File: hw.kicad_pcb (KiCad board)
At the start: 4 copper layers, 75 x 75 mm, 159 parts, among them IC2 ESDALC6V1W5, IC3 ESDALC6V1W5, IC4 QFN50P400X400X80-25N-D, IC5 QFN40P300X300X105-25N-D, J1 RECE.20279.001E.01, J2 RECE.20279.001E.01, J3 78800-0001, J4 AMPHENOL_10164227-1004A1RLF, J5 AMPHENOL_10164227-1004A1RLF, J7 USB4105-GF-A, Q1 BC847CE6327HTSA1, Q2 BC847CE6327HTSA1, Q3 BC847CE6327HTSA1, U11 XDFN8_1P7X1P3_ONS, U2 MOD100_LENA-R8_UBL, U3 STM32H745ZIT6, U4 XDFN8_1P7X1P3_ONS, U5 XDFN8_1P7X1P3_ONS, U8 TS3USB221RSER, Y1 NX3215SA-32.768K-EXS00A-MU000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, Y2 ATX-H11-F-25.000MHz-F25-T

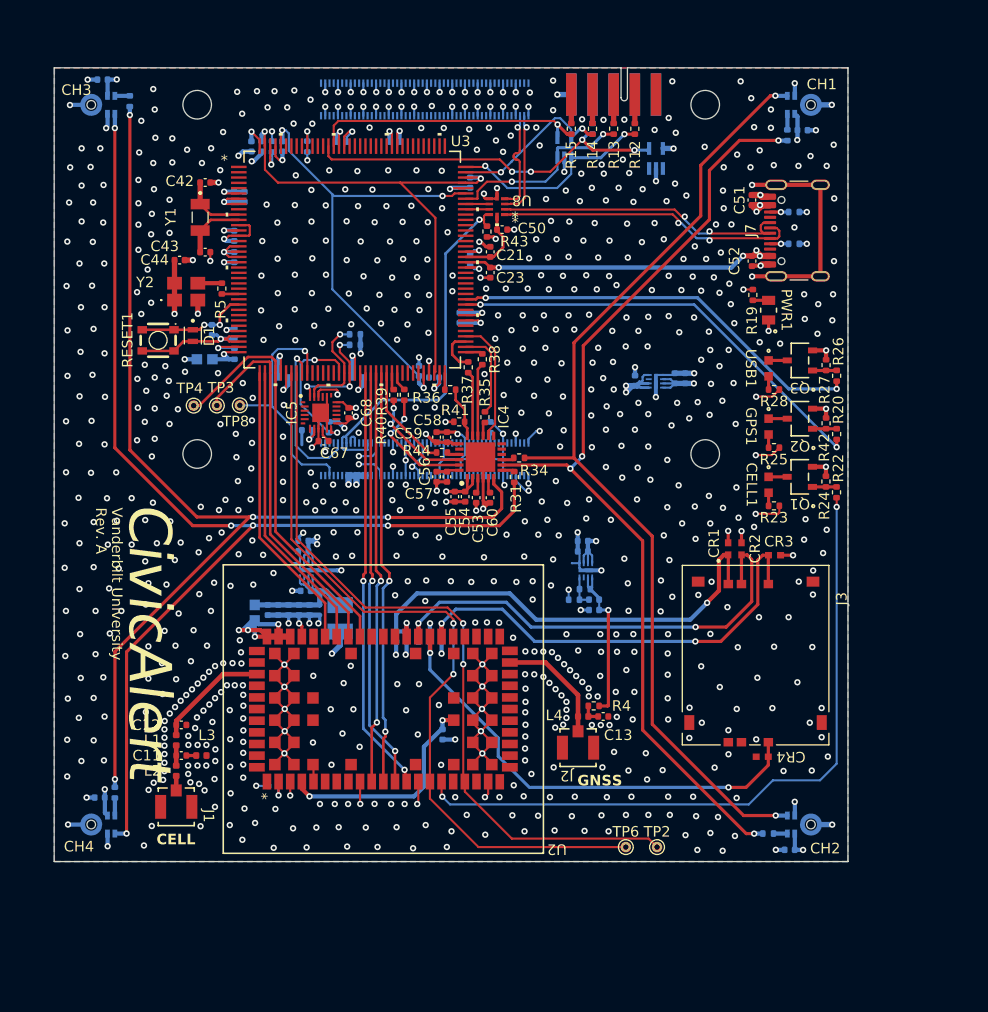
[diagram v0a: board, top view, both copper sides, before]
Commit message: Update for RevB
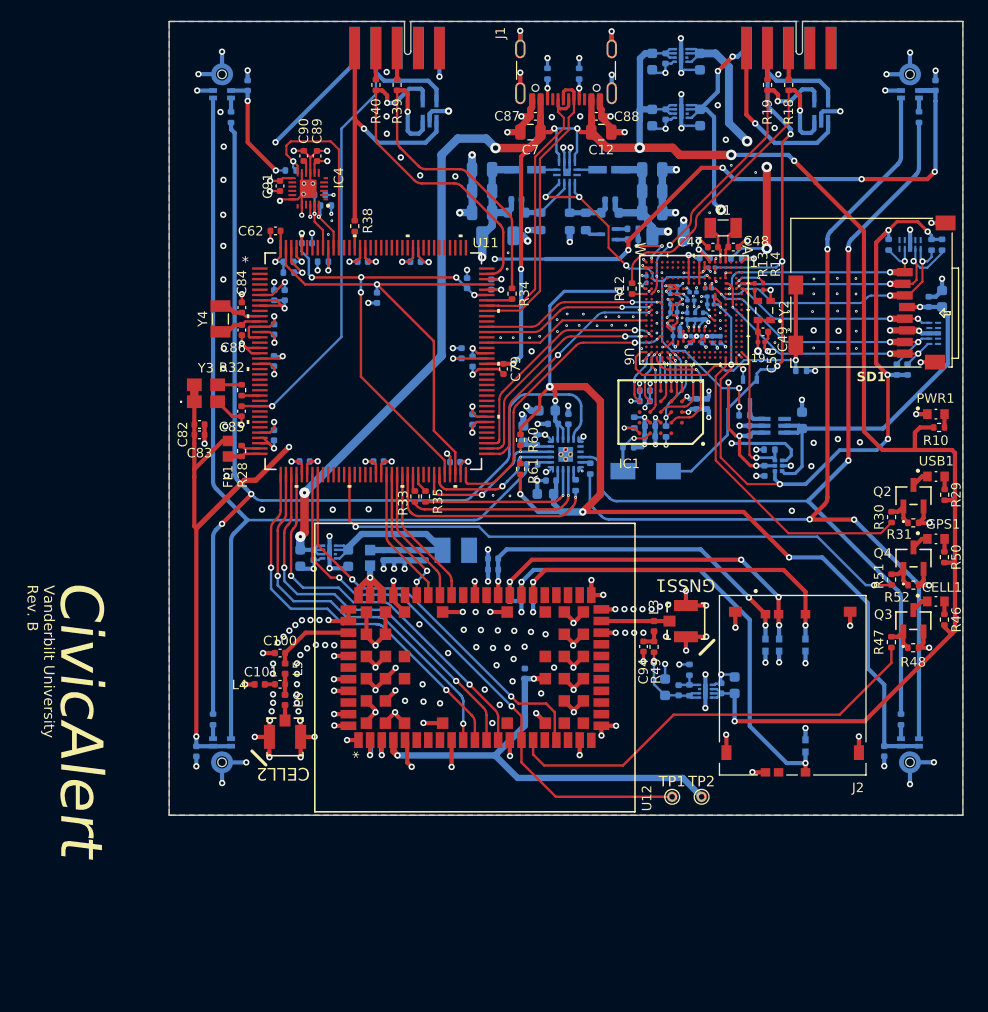
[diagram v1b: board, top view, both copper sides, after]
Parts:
- removed IC5: QFN40P300X300X105-25N-D, CivicAlert:ICM-20948
- removed J3: 78800-0001, CivicAlert:0788000001
- removed J4, J5: AMPHENOL_10164227-1004A1RLF, CivicAlert:10164227-1004A1RLF
- removed J7: USB4105-GF-A, Connector_USB:USB_C_Receptacle_GCT_USB4105-xx-A_16P_TopMnt_Horizontal
- removed Module1: ComputeModule5-CM5, CivicAlert:RPI-CM5IO
- removed RESET1: LS38G2-T, CivicAlert:LS38G2F-T
- removed TP3: GPS_TRIG, TestPoint:TestPoint_THTPad_D1.0mm_Drill0.5mm
- removed TP4: GPS_TP, TestPoint:TestPoint_THTPad_D1.0mm_Drill0.5mm
- removed TP6: GPS_PWR, TestPoint:TestPoint_THTPad_D1.0mm_Drill0.5mm
- removed TP8: RPI_nOFF, TestPoint:TestPoint_THTPad_D1.0mm_Drill0.5mm
- added B2: 009159010061911, CivicAlert:009159010061911, F.Cu at (137.5, 63.4)
- added C100: 1.5p, Capacitor_SMD:C_0402_1005Metric, F.Cu at (122.4, 120.5)
- added C101: 0.5p, Capacitor_SMD:C_0402_1005Metric, F.Cu at (122.4, 123.5)
- added C102: T520B337M006ATE040, CivicAlert:T520B337M006ATE040, B.Cu at (139.0, 110.8)
- added C103: 8.2p, Capacitor_SMD:C_0402_1005Metric, B.Cu at (132.2, 111.3)
- added C104: 15p, Capacitor_SMD:C_0402_1005Metric, B.Cu at (133.2, 111.3)
- added C105: 82p, Capacitor_SMD:C_0402_1005Metric, B.Cu at (134.2, 111.3)
- added C106: 10n, Capacitor_SMD:C_0402_1005Metric, B.Cu at (135.2, 111.3)
- added C107: 0.1u, Capacitor_SMD:C_0402_1005Metric, B.Cu at (136.2, 111.3)
- added C108: 0.1u, Capacitor_SMD:C_0402_1005Metric, B.Cu at (184.3, 66.9)
- added C109: 0.1u, Capacitor_SMD:C_0402_1005Metric, B.Cu at (179.5, 129.8)
- added C110: 0.1u, Capacitor_SMD:C_0402_1005Metric, B.Cu at (119.4, 66.9)
- added C111: 0.1u, Capacitor_SMD:C_0402_1005Metric, B.Cu at (114.5, 129.8)
- added C112: 0.1u, Capacitor_SMD:C_0402_1005Metric, B.Cu at (148.2, 98.9)
- added C113: 10u, Capacitor_SMD:C_0603_1608Metric, B.Cu at (147.6, 97.6)
- added C114: 2.2u, Capacitor_SMD:C_0402_1005Metric, B.Cu at (149.7, 98.4)
- added C115: 10u, Capacitor_SMD:C_0603_1608Metric, B.Cu at (147.5, 105.5)
- added C116: 0.1u, Capacitor_SMD:C_0402_1005Metric, B.Cu at (148.0, 104.2)
- added C117: 0.1u, Capacitor_SMD:C_0402_1005Metric, B.Cu at (146.7, 100.4)
- added C118: 10u, Capacitor_SMD:C_0603_1608Metric, B.Cu at (145.4, 99.8)
- added C70: 0.1u, Capacitor_SMD:C_0402_1005Metric, B.Cu at (124.7, 102.4)
- added C71: 0.1u, Capacitor_SMD:C_0402_1005Metric, B.Cu at (131.7, 102.4)
- added C72: 0.1u, Capacitor_SMD:C_0402_1005Metric, B.Cu at (139.0, 102.5)
- added C73: 0.1u, Capacitor_SMD:C_0402_1005Metric, B.Cu at (140.6, 98.5)
- added C74: 0.1u, Capacitor_SMD:C_0402_1005Metric, B.Cu at (140.6, 93.0)
- added C75: 0.1u, Capacitor_SMD:C_0402_1005Metric, B.Cu at (142.4, 85.7)
- added C76: 4.7u, Capacitor_SMD:C_0402_1005Metric, B.Cu at (131.6, 87.0)
- added C77: 0.1u, Capacitor_SMD:C_0402_1005Metric, B.Cu at (122.9, 86.7)
- added C78: 2.2u, Capacitor_SMD:C_0402_1005Metric, B.Cu at (139.6, 92.2)
- added C79: 4.7u, Capacitor_SMD:C_0402_1005Metric, F.Cu at (143.5, 93.7)
- added C80: 2.2u, Capacitor_SMD:C_0402_1005Metric, B.Cu at (125.0, 81.8)
- added C81: 2.2u, Capacitor_SMD:C_0402_1005Metric, B.Cu at (140.1, 85.6)
- added C82: 10n, Capacitor_SMD:C_0402_1005Metric, F.Cu at (114.8, 98.9)
- added C83: 0.1u, Capacitor_SMD:C_0402_1005Metric, F.Cu at (114.8, 99.9)
- added C84: 3.3p, Capacitor_SMD:C_0402_1005Metric, F.Cu at (118.8, 87.9)
- added C85: 0.1u, Capacitor_SMD:C_0402_1005Metric, F.Cu at (118.8, 97.7)
- added C86: 3.3p, Capacitor_SMD:C_0402_1005Metric, F.Cu at (118.8, 90.0)
- added C87: 0.1u, Capacitor_SMD:C_0402_1005Metric, F.Cu at (146.5, 69.8)
- added C88: 0.1u, Capacitor_SMD:C_0402_1005Metric, F.Cu at (152.3, 69.8)
- added C89: 0.1u, Capacitor_SMD:C_0402_1005Metric, F.Cu at (125.9, 73.6)
- added C9: 10u, Capacitor_SMD:C_0805_2012Metric, B.Cu at (141.5, 78.9)
- added C90: 0.1u, Capacitor_SMD:C_0402_1005Metric, F.Cu at (124.6, 73.6)
- added C91: 0.1u, Capacitor_SMD:C_0402_1005Metric, F.Cu at (122.4, 76.4)
- added C92: 0.1u, Capacitor_SMD:C_0402_1005Metric, B.Cu at (131.5, 129.1)
- added C93: 0.1u, Capacitor_SMD:C_0402_1005Metric, B.Cu at (145.5, 122.5)
- added C94: 0.1u, Capacitor_SMD:C_0402_1005Metric, F.Cu at (156.7, 119.9)
- added C95: 47p, Capacitor_SMD:C_0402_1005Metric, B.Cu at (146.3, 115.1)
- added C96: 47p, Capacitor_SMD:C_0402_1005Metric, B.Cu at (145.2, 115.1)
- added C97: 47p, Capacitor_SMD:C_0402_1005Metric, B.Cu at (144.1, 115.1)
- added C98: 47p, Capacitor_SMD:C_0402_1005Metric, B.Cu at (142.5, 111.6)
- added C99: 0.1u, Capacitor_SMD:C_0402_1005Metric, B.Cu at (142.5, 112.7)
- added CELL2: RECE.20279.001E.01, CivicAlert:RECE.20279.001E.01, F.Cu at (122.9, 128.5)
- added CR5: PESD0402-140, CivicAlert:PESD0402-140_LTF, B.Cu at (172.1, 119.8)
- added GNSS1: RECE.20279.001E.01, CivicAlert:RECE.20279.001E.01, F.Cu at (160.8, 117.5)
- added IC1: MX25UM25645GXDI00-T, CivicAlert:MX25UM25645GXDI00, F.Cu at (158.4, 97.8)
- added L5: 2.7n, Inductor_SMD:L_0402_1005Metric, F.Cu at (122.9, 122.0)
- added L6: 1.2n, Inductor_SMD:L_0402_1005Metric, F.Cu at (122.9, 125.0)
- added Q4: MMBT3904LT3G, CivicAlert:MMBT3904LT3G, F.Cu at (182.3, 111.6)
- added R16: 10k, Resistor_SMD:R_0402_1005Metric, B.Cu at (155.9, 98.8)
- added R17: 10k, Resistor_SMD:R_0402_1005Metric, B.Cu at (158.9, 99.6)
- added R46: 300, Resistor_SMD:R_0402_1005Metric, F.Cu at (185.2, 117.4)
- added R47: 10k, Resistor_SMD:R_0402_1005Metric, F.Cu at (180.2, 119.5)
- added R48: 47k, Resistor_SMD:R_0402_1005Metric, F.Cu at (182.2, 120.0)
- added R49: 33, Resistor_SMD:R_0402_1005Metric, F.Cu at (157.7, 120.0)
- added R50: 300, Resistor_SMD:R_0402_1005Metric, F.Cu at (185.2, 111.5)
- added R51: 10k, Resistor_SMD:R_0402_1005Metric, F.Cu at (180.2, 113.6)
- added R52: 47k, Resistor_SMD:R_0402_1005Metric, F.Cu at (182.2, 114.1)
- added R53: 47, Resistor_SMD:R_0402_1005Metric, B.Cu at (182.8, 69.9)
- added R54: 47, Resistor_SMD:R_0402_1005Metric, B.Cu at (181.1, 126.8)
- added R55: 47, Resistor_SMD:R_0402_1005Metric, B.Cu at (117.8, 69.9)
- added R56: 47, Resistor_SMD:R_0402_1005Metric, B.Cu at (116.1, 126.8)
- added R57: 47, Resistor_SMD:R_0402_1005Metric, B.Cu at (150.3, 104.7)
- added R58: 22, Resistor_SMD:R_0402_1005Metric, B.Cu at (146.2, 102.7)
- added R59: 22, Resistor_SMD:R_0402_1005Metric, B.Cu at (151.7, 103.1)
- added R60: 10k, Resistor_SMD:R_0402_1005Metric, F.Cu at (145.1, 100.4)
- added R61: 10k, Resistor_SMD:R_0402_1005Metric, F.Cu at (145.1, 103.1)
- added SD1: 15882, CivicAlert:15882, F.Cu at (178.3, 86.5)
- added TP1: GPS_PWR, TestPoint:TestPoint_THTPad_D1.0mm_Drill0.5mm, F.Cu at (159.5, 134.1)
- added U1: LTC3315AHV-TRMPBF, CivicAlert:LTC3315AHV, B.Cu at (149.5, 75.1)
- added U10: TPS22919DCKR, CivicAlert:TPS22919DCKR, B.Cu at (169.1, 99.1)
- added U12: LENA-R8001M10-00C, CivicAlert:LENA-R8001M10-00C, F.Cu at (140.8, 121.9)
- added U13: PCMD3140IRTER, CivicAlert:PCMD3140IRTER, B.Cu at (149.4, 101.8)
- added U6: STM32N647L0H3Q, CivicAlert:STM32N647L0H3Q, F.Cu at (161.5, 88.1)
- added U7: HSP051-4M10, CivicAlert:HSP051-4M10, B.Cu at (181.9, 81.9)
- added U9: NX3L1T3157GMZ, CivicAlert:NX3L1T3157GMZ, B.Cu at (169.5, 102.8)
- added Y3: ATX-H11-F-25.000MHz-F25-T, CivicAlert:ATX-H11-F-25_000MHz-F25-T, F.Cu at (115.4, 96.0)
- added Y4: ABS07AIG-32.768KHZ-7-T, CivicAlert:ABS07AIG_32_768KHZ_7_T, F.Cu at (116.8, 89.0)
- C1: value 100n -> 6.8p
- C10, C3: value 100n -> 10u; footprint Capacitor_SMD:C_0402_1005Metric -> Capacitor_SMD:C_0805_2012Metric
- C11: value 0.5p -> 10u; footprint Capacitor_SMD:C_0402_1005Metric -> Capacitor_SMD:C_0805_2012Metric; moved to B.Cu
- C12: value 1.5p -> 10u; footprint Capacitor_SMD:C_0402_1005Metric -> Capacitor_SMD:C_0805_2012Metric
- C13: value 100n -> 1n; moved to B.Cu
- C14, C15, C17: value 47p -> 10u; footprint Capacitor_SMD:C_0402_1005Metric -> Capacitor_SMD:C_0603_1608Metric
- C16: value 47p -> 0.1u
- C18, C24, C64: value 100n -> 0.1u
- C19, C20: value 2.2u -> 10u; footprint Capacitor_SMD:C_0402_1005Metric -> Capacitor_SMD:C_0603_1608Metric
- C2: value 100n -> 4.7p
- C21: value 2.2u -> 0.1u; moved to B.Cu
- C22: value 4.7u -> 10u; footprint Capacitor_SMD:C_0402_1005Metric -> Capacitor_SMD:C_0603_1608Metric
- C23: value 4.7u -> 10u; footprint Capacitor_SMD:C_0402_1005Metric -> Capacitor_SMD:C_0603_1608Metric; moved to B.Cu
- C25, C61: value 100n -> 10u; footprint Capacitor_SMD:C_0402_1005Metric -> Capacitor_SMD:C_0603_1608Metric
- C26, C27, C28, C29, C31, C32, C33, C34, C35, C36, C37, C46: value 100n -> 0.1u; footprint Capacitor_SMD:C_0402_1005Metric -> Capacitor_SMD:C_0201_0603Metric
- C30, C41: value 100n -> 2.2u; footprint Capacitor_SMD:C_0402_1005Metric -> Capacitor_SMD:C_0201_0603Metric
- C38: value 4.7u -> 0.1u; footprint Capacitor_SMD:C_0402_1005Metric -> Capacitor_SMD:C_0201_0603Metric
- C39, C40: value 10u -> 2.2u; footprint Capacitor_SMD:C_0402_1005Metric -> Capacitor_SMD:C_0201_0603Metric
- C4: value 8.2p -> 10u; footprint Capacitor_SMD:C_0402_1005Metric -> Capacitor_SMD:C_0805_2012Metric
- C42, C43: value 1.5p -> 2.2u; footprint Capacitor_SMD:C_0402_1005Metric -> Capacitor_SMD:C_0201_0603Metric; moved to B.Cu
- C44: value 10n -> 4.7u; moved to B.Cu
- C45: value 10u -> 0.1u; footprint Capacitor_SMD:C_0402_1005Metric -> Capacitor_SMD:C_0201_0603Metric
- C47: value 10u -> 3.3p; moved to F.Cu
- C48: value 100n -> 3.3p; moved to F.Cu
- C49: value 100n -> 10n; moved to F.Cu
- C5: value 15p -> 10u; footprint Capacitor_SMD:C_0402_1005Metric -> Capacitor_SMD:C_0805_2012Metric
- C50: value 2.2u -> 0.1u; footprint Capacitor_SMD:C_0402_1005Metric -> Capacitor_SMD:C_0201_0603Metric
- C51, C54, C57, C67, C68: value 100n -> 0.1u; moved to B.Cu
- C52: value 100n -> 4.7u; moved to B.Cu
- C53: value 2.2u -> 4.7u; moved to B.Cu
- C55, C59: value 10u -> 0.1u; moved to B.Cu
- C56: value 10u -> 4.7u; moved to B.Cu
- C58: value 100n -> 10u; footprint Capacitor_SMD:C_0402_1005Metric -> Capacitor_SMD:C_0603_1608Metric; moved to B.Cu
- C6: value 82p -> 47u; footprint Capacitor_SMD:C_0402_1005Metric -> Capacitor_SMD:C_1206_3216Metric
- C60, CR2, CR3, CR4, R24: moved to B.Cu
- C62: value 100n -> 4.7u; moved to F.Cu
- C63, C65: value 10u -> 0.1u
- C66: value 1n -> 0.1u
- C69: value T520B337M006ATE040 -> 0.1u; footprint CivicAlert:T520B337M006ATE040 -> Capacitor_SMD:C_0402_1005Metric
- C7: value 10n -> 10u; footprint Capacitor_SMD:C_0402_1005Metric -> Capacitor_SMD:C_0805_2012Metric; moved to F.Cu
- C8: value 100n -> 47u; footprint Capacitor_SMD:C_0402_1005Metric -> Capacitor_SMD:C_1206_3216Metric
- CELL1, GPS1, USB1: value LTST-C193TBKT-5A -> LTST-C190KGKT; footprint CivicAlert:LTST-C193TBKT-5A -> CivicAlert:LTST-C190KGKT
- CR1: value PESD0402-140 -> BAT854AW; footprint CivicAlert:PESD0402-140_LTF -> CivicAlert:BAT854AW,115; moved to B.Cu
- D1: value NSPM2051MUT5G -> B140Q-13-F; footprint CivicAlert:NSPM2051MUT5G -> CivicAlert:B140Q-13-F; moved to B.Cu
- FL1: value BLM18EG221SN1D -> FCM 1608KF-601T03; footprint CivicAlert:BLM18EG221SN1D -> CivicAlert:FCM1608KF-601T03; moved to F.Cu
- FL2: value FCM 1608KF-601T03 -> BLM18EG221SN1D; footprint CivicAlert:FCM1608KF-601T03 -> CivicAlert:BLM18EG221SN1D
- IC4: value QFN50P400X400X80-25N-D -> ICM-20948; footprint CivicAlert:PCMD3180IRTWT -> CivicAlert:ICM-20948
- J1: value RECE.20279.001E.01 -> USB4105-GF-A; footprint CivicAlert:RECE.20279.001E.01 -> Connector_USB:USB_C_Receptacle_GCT_USB4105-xx-A_16P_TopMnt_Horizontal
- J2: value RECE.20279.001E.01 -> 78800-0001; footprint CivicAlert:RECE.20279.001E.01 -> CivicAlert:0788000001
- L1: value 2.7n -> IHLP1212BZERR88M11; footprint Inductor_SMD:L_0402_1005Metric -> CivicAlert:IHLP1212BZERR88M11; moved to B.Cu
- L2: value 1.2n -> IHLP1212BZER1R5M11; footprint Inductor_SMD:L_0402_1005Metric -> CivicAlert:IHLP1212BZER1R5M11; moved to B.Cu
- L3: value 3.4n -> 120n
- L4: value 120n -> 3.4n
- PWR1: value LTST-C170KRKT -> LTST-C190KGKT; footprint CivicAlert:LTST-C170KRKT -> CivicAlert:LTST-C190KGKT
- Q1: value BC847CE6327HTSA1 -> SI1062X-T1-GE3; footprint CivicAlert:BC847CE6327HTSA1 -> CivicAlert:SI1062X-T1-GE3; moved to B.Cu
- Q2, Q3: value BC847CE6327HTSA1 -> MMBT3904LT3G; footprint CivicAlert:BC847CE6327HTSA1 -> CivicAlert:MMBT3904LT3G
- R1: value 50 -> 1M
- R10: value 10k -> 300; moved to F.Cu
- R13: footprint Resistor_SMD:R_0402_1005Metric -> Resistor_SMD:R_0201_0603Metric
- R14: value 22 -> 1k; footprint Resistor_SMD:R_0402_1005Metric -> Resistor_SMD:R_0201_0603Metric
- R15: value 22 -> 10k; moved to B.Cu
- R18: moved to F.Cu
- R19: value 250 -> 22
- R2: value 50 -> 150k
- R20, R22: value 10k -> 47k; moved to B.Cu
- R21: value 8.2k -> 10k
- R23, R25: value 500 -> 47k; moved to B.Cu
- R26: value 10k -> 100k; moved to B.Cu
- R27: value 47k -> 10k; moved to B.Cu
- R28: value 500 -> 47
- R29: value 5.1k -> 300; moved to F.Cu
- R3: value 50 -> 226k; footprint Resistor_SMD:R_0402_1005Metric -> Resistor_SMD:R_0603_1608Metric
- R30: value 5.1k -> 10k; moved to F.Cu
- R31: value 22 -> 47k
- R32: value 50 -> 22; moved to F.Cu
- R33: value 50 -> 47; moved to F.Cu
- R35: value 50 -> 47
- R36, R37, R44: value 50 -> 10k; moved to B.Cu
- R38, R39, R40: value 50 -> 22
- R4: value 33 -> 887k; footprint Resistor_SMD:R_0402_1005Metric -> Resistor_SMD:R_0603_1608Metric; moved to B.Cu
- R41: value 10k -> 5.1k; moved to B.Cu
- R42: value 47k -> 5.1k; moved to B.Cu
- R43: value 100k -> 10k; moved to B.Cu
- R45: value 1k -> 10k
- R5: value 50 -> 140k; footprint Resistor_SMD:R_0402_1005Metric -> Resistor_SMD:R_0603_1608Metric; moved to B.Cu
- R6: value 5.1k -> 97.6k; footprint Resistor_SMD:R_0402_1005Metric -> Resistor_SMD:R_0603_1608Metric
- R7: value 10k -> 261k; footprint Resistor_SMD:R_0402_1005Metric -> Resistor_SMD:R_0603_1608Metric
- R8: value 10k -> 62k
- R9: value 10k -> 91k
- TP2: value GPS_nRST -> GPS_VINT
- U11: value XDFN8_1P7X1P3_ONS -> STM32H745ZIT6; footprint CivicAlert:NCP186BMX185TAG -> CivicAlert:STM32H745ZIT6; moved to F.Cu
- U2: value MOD100_LENA-R8_UBL -> NCP186AMX180TAG; footprint CivicAlert:LENA-R8001M10-00C -> CivicAlert:NCP186AMX; moved to B.Cu
- U3: value STM32H745ZIT6 -> NCP186AMX390TAG; footprint CivicAlert:STM32H745ZIT6 -> CivicAlert:NCP186AMX; moved to B.Cu
- U4: value XDFN8_1P7X1P3_ONS -> NCP186AMX180TAG; footprint CivicAlert:NCP186AMX390TAG -> CivicAlert:NCP186AMX
- U5: value XDFN8_1P7X1P3_ONS -> NCP186AMX330TAG; footprint CivicAlert:NCP186BMX185TAG -> CivicAlert:NCP186AMX
- U8: value TS3USB221RSER -> HSP051-4M10; footprint CivicAlert:TS3USB221RSER -> CivicAlert:HSP051-4M10; moved to B.Cu
- Y1: value NX3215SA-32.768K-EXS00A-MU00003 -> ABS07AIG-32.768KHZ-7-T; footprint CivicAlert:NX3215SA-32_768K-EXS00A-MU0000 -> CivicAlert:ABS07AIG_32_768KHZ_7_T
- Y2: value ATX-H11-F-25.000MHz-F25-T -> KC2016Z48.0000C15XXK; footprint CivicAlert:ATX-H11-F-25_000MHz-F25-T -> CivicAlert:KC2016Z48.0000C15XXK
- moved J1 79.6 mm to (149.4, 64.5)
- moved C61 73.5 mm to (171.7, 98.5), turned to 90 degrees
- moved C12 68.6 mm to (152.8, 71.3)
- moved L1 67.7 mm to (153.5, 74.9), turned to 0 degrees
- moved C2 66.7 mm to (144.7, 77.7)
- moved L2 65.7 mm to (145.6, 74.9), turned to 180 degrees
- moved R10 65.3 mm to (184.7, 99.2), turned to 180 degrees
- moved C11 62.2 mm to (141.5, 74.9)
- moved U4 60.2 mm to (160.3, 64.1), turned to 180 degrees
- moved C10 59.6 mm to (141.5, 76.9)
- moved R2 58.5 mm to (155.8, 80.5)
- moved C62 56.1 mm to (122.0, 80.7), turned to 0 degrees
- moved Y2 54.6 mm to (168.2, 88.2), turned to 180 degrees
- moved C5 54.6 mm to (157.6, 74.9), turned to 0 degrees
- moved C4 53.7 mm to (157.6, 76.9), turned to 0 degrees
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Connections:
- B1 pad 10: MCU_VCC -> VCC_AI_IO
- B1 pad 2: Net-(B1-JTDI) -> unconnected-(B1-JTDI-Pad2)
- B1 pad 5: Net-(B1-JTDO/SWO) -> AI_SWO
- B1 pad 9: Net-(B1-NRST) -> AI_NRST
- C1 pad 1: MCU_VCC -> Net-(U1-FB1)
- C1 pad 2: GND -> VCC_AI_CORE
- C10 pad 1: Net-(U2-V_BCKP) -> VCC_MCU
- C11 pad 1: Net-(C11-Pad1) -> VCC_MCU
- C11 pad 2: Net-(C11-Pad2) -> GND
- C12 pad 2: Net-(U2-ANT) -> VCC_5V
- C13 pad 1: GND -> VCC_GPS_ANT
- C13 pad 2: Net-(C13-Pad2) -> Net-(U2-FB/ADJ)
- C14 pad 1: GND -> VCC_GPS_ANT
- C14 pad 2: SIM_CLK -> GND
- C15 pad 1: GND -> VCC_5V
- C15 pad 2: SIM_IO -> GND
- C16 pad 1: GND -> VCC_5V
- C16 pad 2: SIM_RST -> GND
- C17 pad 1: GND -> VCC_5V
- C17 pad 2: SIM_VCC -> GND
- C18 pad 1: GND -> VCC_5V
- C18 pad 2: SIM_VCC -> GND
- C19 pad 1: Net-(C19-Pad1) -> VCC_CELL_GPS
- C2 pad 1: MCU_VCC -> Net-(U1-FB2)
- C2 pad 2: GND -> VCC_MCU
- C20 pad 1: Net-(C19-Pad1) -> VCC_5V
- C21 pad 1: VCC_3V3 -> VCC_5V
- C22 pad 1: MCU_VCC -> VCC_AI_ON
- C24 pad 1: GND -> VCC_5V
- C24 pad 2: MCU_VCC -> GND
- C25 pad 1: MCU_VCC -> VCC_AI_IO
- C26 pad 1: MCU_VCC -> AI_NRST
- C27 pad 1: MCU_VCC -> GND
- C27 pad 2: GND -> VCC_AI_IO
- C28 pad 1: MCU_VCC -> GND
- C28 pad 2: GND -> VCC_AI_IO
- C29 pad 1: MCU_VCC -> GND
- C29 pad 2: GND -> VCC_AI_IO
- C3 pad 1: GPS_VINT -> VCC_AI_CORE
- C30 pad 1: MCU_VCC -> VCC_AI_CORE
- C31 pad 1: MCU_VCC -> GND
- C31 pad 2: GND -> VCC_AI_ON
- C32 pad 2: MCU_VCC -> VCC_AI_ON
- C33 pad 2: MCU_VCC -> VCC_AI_ON
- C34 pad 2: MCU_VCC -> VCC_AI_ON
- C35 pad 1: GND -> VCC_AI_ON
- C35 pad 2: MCU_VCC -> GND
- C36 pad 1: GND -> VCC_AI_ON
- C36 pad 2: MCU_VCC -> GND
- C37 pad 1: GND -> VDDIO_SD
- C37 pad 2: MCU_VCC -> GND
- C38 pad 1: GND -> VDDIO_SD
- C38 pad 2: MCU_VCC -> GND
- C39 pad 1: VCC_5V -> VCC_AI_CORE
- C4 pad 1: GPS_VCC -> VCC_AI_CORE
- C40 pad 1: MCU_VCC -> VCC_AI_CORE
- C41 pad 1: VCC_5V -> VCC_AI_CORE
- C42 pad 1: Net-(U3A-PC14-OSC32_IN) -> VCC_AI_CORE
- C43 pad 1: Net-(U3A-PC15-OSC32_OUT) -> VCC_AI_CORE
- C44 pad 1: MCU_VCC -> Net-(U6D-V08CAP)
- C45 pad 1: VCC_5V -> GND
- C45 pad 2: GND -> VCC_AI_ON
- C46 pad 1: VCC_5V -> VCC_MCU
- C47 pad 1: GPS_VCC -> Net-(U6A-PC14-OSC32_IN)
- C48 pad 1: GND -> Net-(U6A-PC15-OSC32_OUT)
- C48 pad 2: MCU_VCC -> GND
- C49 pad 1: Net-(U3B-NRST) -> VCC_AI_ON
- C5 pad 1: GPS_VCC -> VCC_AI_CORE
- C50 pad 1: GND -> VCC_AI_ON
- C50 pad 2: VCC_3V3 -> GND
- C51 pad 1: VCC_5V -> VCC_AI_ON
- C52 pad 1: VCC_5V -> VCC_AI_ON
- C53 pad 1: Net-(IC4-VREF) -> VCC_AI_ON
- C54 pad 1: MCU_VCC -> VCC_AI_ON
- C55 pad 1: MCU_VCC -> VCC_AI_ON
- C56 pad 1: Net-(IC4-DREG) -> VCC_AI_ON
- C57 pad 1: Net-(IC4-DREG) -> GND
- C57 pad 2: GND -> VCC_SD
- C58 pad 1: MCU_VCC -> GND
- C58 pad 2: GND -> VCC_SD
- C59 pad 1: MCU_VCC -> GND
- C59 pad 2: GND -> VCC_AI_IO
- C6 pad 1: GPS_VCC -> VCC_AI_CORE
- C60 pad 2: Net-(IC4-MICBIAS) -> VCC_AI_IO
- C61 pad 1: MCU_VCC -> VCC_SD
- C62 pad 1: MCU_VCC -> GND
- C62 pad 2: GND -> VCC_MCU
- C63 pad 1: VCC_5V -> GND
- C63 pad 2: GND -> VCC_MCU
- C64 pad 1: VCC_5V -> GND
- C64 pad 2: GND -> VCC_MCU
- C65 pad 1: ANTENNA_VCC -> GND
- C65 pad 2: GND -> VCC_MCU
- C66 pad 1: ANTENNA_VCC -> GND
- C66 pad 2: Net-(U11-FB/ADJ) -> VCC_MCU
- C67 pad 2: Net-(IC5-REGOUT) -> VCC_MCU
- C68 pad 2: MCU_VCC -> VCC_MCU
- C69 pad 1: GPS_VCC -> VCC_MCU
- C7 pad 1: GPS_VCC -> VCC_5V
- C8 pad 1: GPS_VCC -> VCC_MCU
- CH1 pad 2: MCU_VCC -> VCC_MCU
- CH2 pad 2: MCU_VCC -> VCC_MCU
- CH2 pad 4: MCU_VCC -> VCC_MCU
- CH3 pad 2: MCU_VCC -> VCC_MCU
- CH4 pad 2: MCU_VCC -> VCC_MCU
- CH4 pad 4: MCU_VCC -> VCC_MCU
- CR1 pad 1: SIM_VCC -> SD_CARD_EN
- CR1 pad 2: GND -> AI_NRST
- CR2 pad 1: SIM_RST -> SIM_IO
- CR3 pad 1: SIM_CLK -> SIM_VCC
- CR4 pad 1: SIM_IO -> SIM_RST
- FL1 pad 1: Net-(FL1-Pad1) -> VCC_MCU
- FL1 pad 2: GPS_VCC -> Net-(U11C-VDDA)
- FL2 pad 1: MCU_VCC -> Net-(FL2-Pad1)
- FL2 pad 2: Net-(U3C-VDDA) -> VCC_CELL_GPS
- IC2 pad 1: JTDI -> AI_SWO
- IC2 pad 3: SWDIO -> AI_SWDIO
- IC2 pad 4: SWO -> AI_SWCLK
- IC2 pad 5: SWDCLK -> AI_NRST
- IC3 pad 1: unconnected-(IC3-I/01-Pad1) -> MCU_SWO
- IC3 pad 3: unconnected-(IC3-I/02-Pad3) -> MCU_SWDIO
- IC3 pad 4: JTAG_RST -> MCU_SWDCLK
- IC3 pad 5: VCC_5V -> MCU_NRST
- IC4 pad 1: MCU_VCC -> unconnected-(IC4-NC_1-Pad1)
- IC4 pad 10: unconnected-(IC4-PDMDIN3_GPI3-Pad10) -> Net-(IC4-REGOUT)
- IC4 pad 11: unconnected-(IC4-PDMCLK3_GPO3-Pad11) -> GND
- IC4 pad 12: unconnected-(IC4-PDMDIN4_GPI4-Pad12) -> IMU_INT
- IC4 pad 13: unconnected-(IC4-PDMCLK4_GPO4-Pad13) -> VCC_MCU
- IC4 pad 14: MICS_nRESET -> unconnected-(IC4-NC_7-Pad14)
- IC4 pad 15: Net-(IC4-ADDR1_MISO) -> unconnected-(IC4-NC_8-Pad15)
- IC4 pad 16: MICS_SCLK -> unconnected-(IC4-NC_9-Pad16)
- IC4 pad 17: MICS_MOSI -> unconnected-(IC4-NC_10-Pad17)
- IC4 pad 18: MICS_CS -> GND
- IC4 pad 19: MCU_VCC -> unconnected-(IC4-RESV_1-Pad19)
- IC4 pad 2: MCU_VCC -> unconnected-(IC4-NC_2-Pad2)
- IC4 pad 20: unconnected-(IC4-GPIO1-Pad20) -> GND
- IC4 pad 21: Net-(IC4-SDOUT) -> unconnected-(IC4-AUX_DA-Pad21)
- IC4 pad 22: AUDIO_CLK -> VCC_MCU
- IC4 pad 23: AUDIO_FSYNC -> IMU_SCL
- IC4 pad 24: Net-(IC4-DREG) -> IMU_SDA
- IC4 pad 3: Net-(IC4-VREF) -> unconnected-(IC4-NC_3-Pad3)
- IC4 pad 4: GND -> unconnected-(IC4-NC_4-Pad4)
- IC4 pad 5: Net-(IC4-MICBIAS) -> unconnected-(IC4-NC_5-Pad5)
- IC4 pad 6: MIC_DATA3_4 -> unconnected-(IC4-NC_6-Pad6)
- IC4 pad 7: Net-(IC4-PDMCLK1_GPO1) -> unconnected-(IC4-AUX_CL-Pad7)
- IC4 pad 8: MIC_DATA1_2 -> VCC_MCU
- IC4 pad 9: Net-(IC4-PDMCLK2_GPO2) -> GND
- L1 pad 1: Net-(U2-ANT) -> Net-(U1-SW1)
- L1 pad 2: Net-(C11-Pad2) -> VCC_AI_CORE
- L2 pad 1: Net-(C11-Pad2) -> Net-(U1-SW2)
- L2 pad 2: Net-(J1-SIGNAL) -> VCC_MCU
- L3 pad 1: Net-(C11-Pad1) -> Net-(GNSS1-SIGNAL)
- L3 pad 2: GND -> Net-(C94-Pad2)
- L4 pad 1: Net-(J2-SIGNAL) -> Net-(C101-Pad1)
- L4 pad 2: Net-(C13-Pad2) -> GND
- Q1 pad 3: Net-(CELL1-Pad1) -> Net-(Q1-Pad3)
- Q2 pad 3: Net-(GPS1-Pad1) -> Net-(Q2-Pad3)
- Q3 pad 3: Net-(Q3-Pad3) -> Net-(CELL1-PadC)
- R1 pad 1: MIC_DATA1_2 -> GND
- R1 pad 2: Net-(CH1-DATA) -> AI_OVERDRIVE
- R10 pad 1: Net-(U3B-BOOT0) -> Net-(PWR1-PadA)
- R10 pad 2: GND -> VCC_5V
- R11 pad 1: Net-(U3B-PDR_ON) -> Net-(U6C-PDR_ON)
- R11 pad 2: MCU_VCC -> VCC_AI_ON
- R12 pad 1: JTDI -> AI_SWDIO
- R12 pad 2: Net-(B1-JTDI) -> Net-(U6A-PA13)
- R13 pad 1: SWDIO -> Net-(Y2-OUTPUT)
- R13 pad 2: Net-(B1-JTMS/SWDIO) -> Net-(U6B-PH0-OSC_IN)
- R14 pad 1: SWDCLK -> GND
- R14 pad 2: Net-(B1-JCLK/SWCLK) -> Net-(U6B-PH1-OSC_OUT)
- R15 pad 1: SWO -> Net-(D1-A)
- R15 pad 2: Net-(B1-JTDO/SWO) -> VCC_AI_ON
- R18 pad 1: JTAG_RST -> AI_SWDIO
- R18 pad 2: Net-(B1-NRST) -> Net-(B1-JTMS/SWDIO)
- R19 pad 1: Net-(PWR1-Pad2) -> AI_SWCLK
- R19 pad 2: VCC_5V -> Net-(B1-JCLK/SWCLK)
- R2 pad 1: MIC_DATA1_2 -> Net-(Q1-Pad1)
- R2 pad 2: Net-(CH2-DATA) -> AI_OVERDRIVE
- R20 pad 1: LED_GPS_STATUS -> SD_DAT3
- R20 pad 2: Net-(Q2-Pad1) -> VDDIO_SD
- R21 pad 1: GND -> SD_CMD
- R21 pad 2: Net-(U11-FB/ADJ) -> VDDIO_SD
- R22 pad 1: LED_NETWORK -> SD_DAT0
- R22 pad 2: Net-(Q1-Pad1) -> VDDIO_SD
- R23 pad 1: Net-(CELL1-Pad2) -> SD_DAT1
- R23 pad 2: VCC_5V -> VDDIO_SD
- R24 pad 1: Net-(Q1-Pad1) -> VDDIO_SD
- R24 pad 2: GND -> SD_DAT2
- R25 pad 1: Net-(GPS1-Pad2) -> VCC_AI_ON
- R25 pad 2: VCC_5V -> SD_CARD_DETECT
- R26 pad 1: LED_USB_STATUS -> SD_PWR_SELECT
- R26 pad 2: Net-(Q3-Pad1) -> GND
- R27 pad 1: GND -> AI_PWR_ON
- R27 pad 2: Net-(Q3-Pad1) -> Net-(U10-ON)
- R28 pad 1: Net-(R28-Pad1) -> Net-(U11C-VDDA)
- R28 pad 2: VCC_5V -> Net-(U11C-VREF+)
- R29 pad 1: GND -> Net-(R29-Pad1)
- R29 pad 2: Net-(J7-CC1) -> VCC_5V
- R3 pad 1: Net-(U3C-VDDA) -> GND
- R3 pad 2: Net-(U3C-VREF+) -> Net-(U1-FB1)
- R30 pad 1: GND -> LED_MCU_STATUS
- R30 pad 2: Net-(J7-CC2) -> Net-(Q2-Pad1)
- R31 pad 1: Net-(IC4-PDMCLK1_GPO1) -> GND
- R31 pad 2: MIC_CLK3_4 -> Net-(Q2-Pad1)
- R32 pad 1: MIC_DATA3_4 -> Net-(U11B-PH0-OSC_IN)
- R32 pad 2: Net-(CH3-DATA) -> Net-(Y3-OUTPUT)
- R33 pad 1: MIC_DATA3_4 -> AUDIO_CLK
- R33 pad 2: Net-(CH4-DATA) -> Net-(U11B-PE12)
- R34 pad 1: Net-(IC4-PDMCLK2_GPO2) -> MCU_SWDIO
- R34 pad 2: MIC_CLK1_2 -> Net-(U11A-PA13)
- R35 pad 1: Net-(IC4-ADDR1_MISO) -> AUDIO_FSYNC
- R35 pad 2: MICS_MISO -> Net-(U11B-PE13)
- R36 pad 1: Net-(U3A-PB12) -> Net-(U11B-BOOT0)
- R36 pad 2: MICS_CS -> GND
- R37 pad 1: Net-(U3A-PB15) -> Net-(U11B-PDR_ON)
- R37 pad 2: MICS_MOSI -> VCC_MCU
- R38 pad 1: Net-(U3A-PB13) -> MCU_SWO
- R38 pad 2: MICS_SCLK -> Net-(U11A-PB3)
- R39 pad 1: AUDIO_CLK -> MCU_SWDIO
- R39 pad 2: Net-(U3B-PE12) -> Net-(B2-JTMS/SWDIO)
- R4 pad 1: Net-(C13-Pad2) -> Net-(Q1-Pad3)
- R4 pad 2: ANTENNA_VCC -> Net-(U1-FB1)
- R40 pad 1: AUDIO_FSYNC -> MCU_SWDCLK
- R40 pad 2: Net-(U3B-PE13) -> Net-(B2-JCLK/SWCLK)
- R41 pad 1: MCU_VCC -> GND
- R41 pad 2: MICS_CS -> Net-(J1-CC1)
- R42 pad 1: Net-(Q2-Pad1) -> GND
- R42 pad 2: GND -> Net-(J1-CC2)
- R43 pad 1: RPI_DETECT -> VCC_MCU
- R43 pad 2: GND -> IMU_SDA
- R44 pad 1: Net-(IC4-SDOUT) -> IMU_SCL
- R44 pad 2: AUDIO_SD -> VCC_MCU
- R45 pad 1: Net-(Module1A-EEPROM_nWP) -> VCC_MCU
- R45 pad 2: GND -> IMU_INT
- R5 pad 1: Net-(U3B-PH0-OSC_IN) -> VCC_AI_CORE
- R5 pad 2: Net-(Y2-OUTPUT) -> Net-(U1-FB1)
- R6 pad 1: Net-(U11-FB/ADJ) -> Net-(U1-FB2)
- R6 pad 2: ANTENNA_VCC -> GND
- R7 pad 1: MCU_VCC -> VCC_MCU
- R7 pad 2: IMU_SDA -> Net-(U1-FB2)
- R8 pad 1: IMU_SCL -> Net-(U2-FB/ADJ)
- R8 pad 2: MCU_VCC -> VCC_GPS_ANT
- R9 pad 1: MCU_VCC -> GND
- R9 pad 2: IMU_INT -> Net-(U2-FB/ADJ)
- TP2 pad 1: GPS_NRESET -> GPS_VINT
- U11 pad 1: ANTENNA_VCC -> unconnected-(U11B-PE2-Pad1)
- U11 pad 2: ANTENNA_VCC -> unconnected-(U11B-PE3-Pad2)
- U11 pad 4: Net-(U11-FB/ADJ) -> unconnected-(U11B-PE5-Pad4)
- U11 pad 5: GND -> unconnected-(U11B-PE6-Pad5)
- U11 pad 6: VCC_5V -> GND
- U11 pad 7: VCC_5V -> VCC_MCU
- U11 pad 8: VCC_5V -> VCC_MCU
- U11 pad 9: GND -> unconnected-(U11A-PC13-Pad9)
- U2 pad 1: GND -> VCC_GPS_ANT
- U2 pad 2: Net-(U2-V_BCKP) -> VCC_GPS_ANT
- U2 pad 3: GND -> unconnected-(U2-N/C-Pad3)
- U2 pad 4: GPS_VINT -> Net-(U2-FB/ADJ)
- U2 pad 6: unconnected-(U2-DSR-Pad6) -> VCC_5V
- U2 pad 7: unconnected-(U2-RI-Pad7) -> VCC_5V
- U2 pad 8: unconnected-(U2-DCD-Pad8) -> VCC_5V
- U3 pad 1: unconnected-(U3B-PE2-Pad1) -> VCC_CELL_GPS
- U3 pad 2: unconnected-(U3B-PE3-Pad2) -> VCC_CELL_GPS
- U3 pad 4: unconnected-(U3B-PE5-Pad4) -> VCC_CELL_GPS
- U3 pad 5: unconnected-(U3B-PE6-Pad5) -> GND
- U3 pad 6: GND -> VCC_5V
- U3 pad 7: MCU_VCC -> VCC_5V
- U3 pad 8: MCU_VCC -> VCC_5V
- U3 pad 9: unconnected-(U3A-PC13-Pad9) -> GND
- U4 pad 1: GPS_VCC -> VCC_AI_ON
- U4 pad 2: GPS_VCC -> VCC_AI_ON
- U4 pad 4: GPS_VCC -> VCC_AI_ON
- U5 pad 1: MCU_VCC -> VCC_AI_IO
- U5 pad 2: MCU_VCC -> VCC_AI_IO
- U5 pad 4: MCU_VCC -> VCC_AI_IO
- U8 pad 1: USB_DEBUG_D- -> SD_DAT1
- U8 pad 10: VCC_3V3 -> unconnected-(U8-NC__3-Pad10)
- U8 pad 2: USB_DEBUG_D+ -> SD_DAT0
- U8 pad 3: USB_RPI_D- -> GND
- U8 pad 4: USB_RPI_D+ -> unconnected-(U8-I/O_3-Pad4)
- U8 pad 5: GND -> SD_CLK
- U8 pad 6: GND -> unconnected-(U8-NC-Pad6)
- U8 pad 7: USB_MCU_D+ -> unconnected-(U8-NC__1-Pad7)
- U8 pad 8: USB_MCU_D- -> GND
- U8 pad 9: RPI_DETECT -> unconnected-(U8-NC__2-Pad9)
- Y1 pad 1: Net-(U3A-PC14-OSC32_IN) -> Net-(U6A-PC14-OSC32_IN)
- Y1 pad 2: Net-(U3A-PC15-OSC32_OUT) -> Net-(U6A-PC15-OSC32_OUT)
- Y2 pad 1: MCU_VCC -> VCC_AI_ON
- Y2 pad 4: MCU_VCC -> VCC_AI_ON
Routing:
- net VCC_MCU: track 0.00 -> 358.3 mm, vias 0 -> 38
- net VCC_5V: track 66.0 -> 236.3 mm, vias 17 -> 11
- net MCU_VCC: track 130.9 -> 0.00 mm, vias 34 -> 0
- net VCC_AI_ON: track 0.00 -> 122.6 mm, vias 0 -> 18
- net GND: track 310.5 -> 384.2 mm, vias 859 -> 355
- net VDDIO_SD: track 0.00 -> 67.9 mm, vias 0 -> 7
- net AI_NRST: track 0.00 -> 61.0 mm, vias 0 -> 4
- net VCC_AI_IO: track 0.00 -> 60.5 mm, vias 0 -> 11
- net MCU_NRST: track 0.00 -> 49.1 mm, vias 0 -> 1
- net Net-(C19-Pad1): track 46.9 -> 0.00 mm, vias 3 -> 0
- net Net-(C80-Pad1): track 0.00 -> 45.1 mm, vias 0 -> 6
- net AI_PWR_ON: track 0.00 -> 41.6 mm, vias 0 -> 6
- net LED_USB_STATUS: track 39.4 -> 0.00 mm, vias 2 -> 0
- net RPI_DETECT: track 36.6 -> 0.00 mm, vias 1 -> 0
- net JTAG_RST: track 34.8 -> 0.00 mm, vias 4 -> 0
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- added copper zone on In2.Cu, net VCC_AI_CORE
- added copper zone on In2.Cu, net VCC_MCU
- removed copper zone on In2.Cu, net MCU_VCC
- removed copper zone on In2.Cu, net VCC_5V
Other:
- outline, holes or cut-outs redrawn
- board text added: "Rev. B"
- board text removed: "CELL"
- board text removed: "GNSS"
- board text removed: "Rev. A"
